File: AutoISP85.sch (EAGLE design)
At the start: 4 parts, among them J1 MCU, J2 BOARD, U1 ATTINY85, U2 BOARD

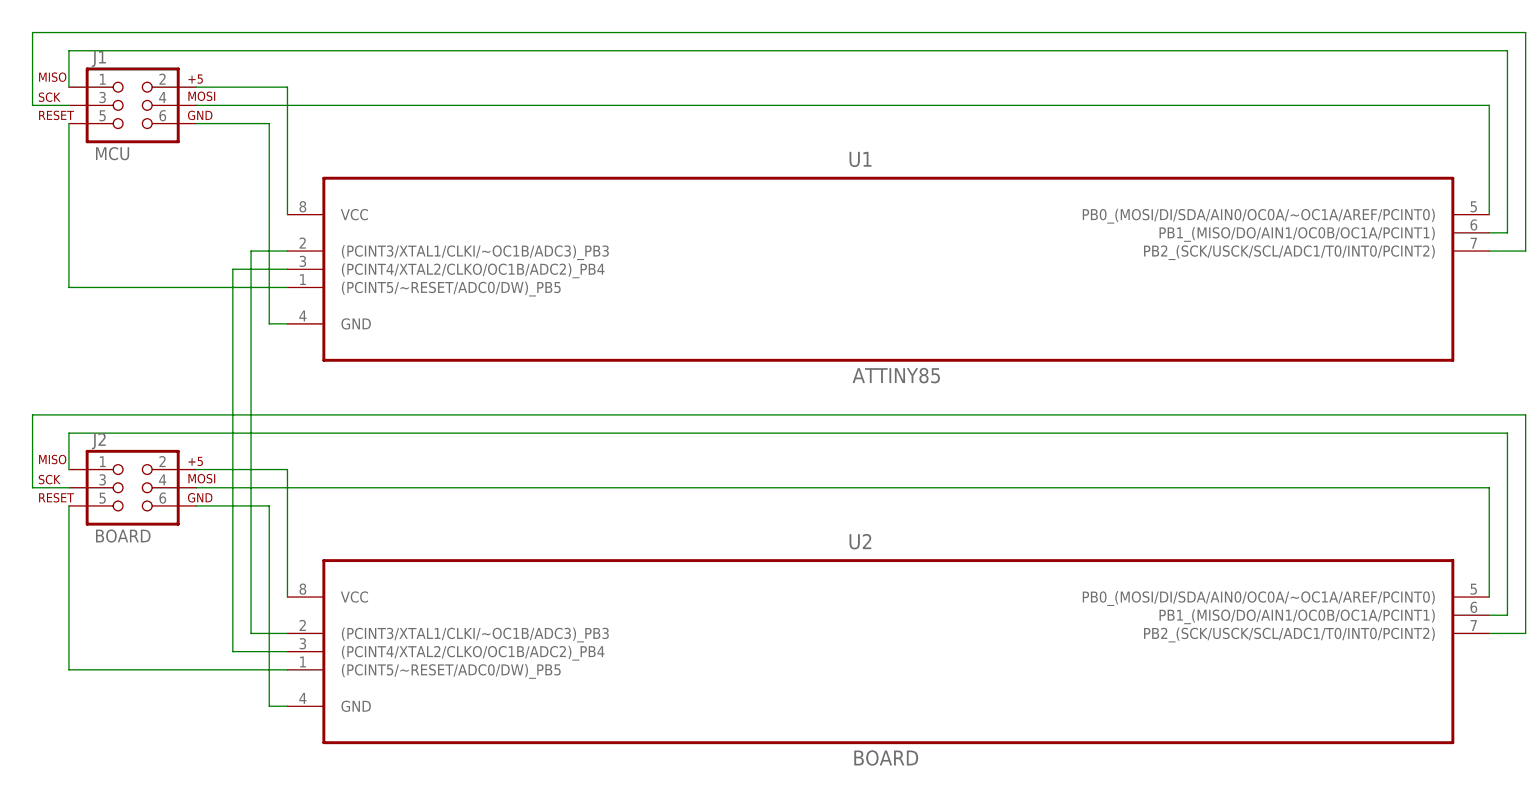
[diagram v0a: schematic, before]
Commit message: Revise boards for better labelling and sane orientation, add AutoISP328
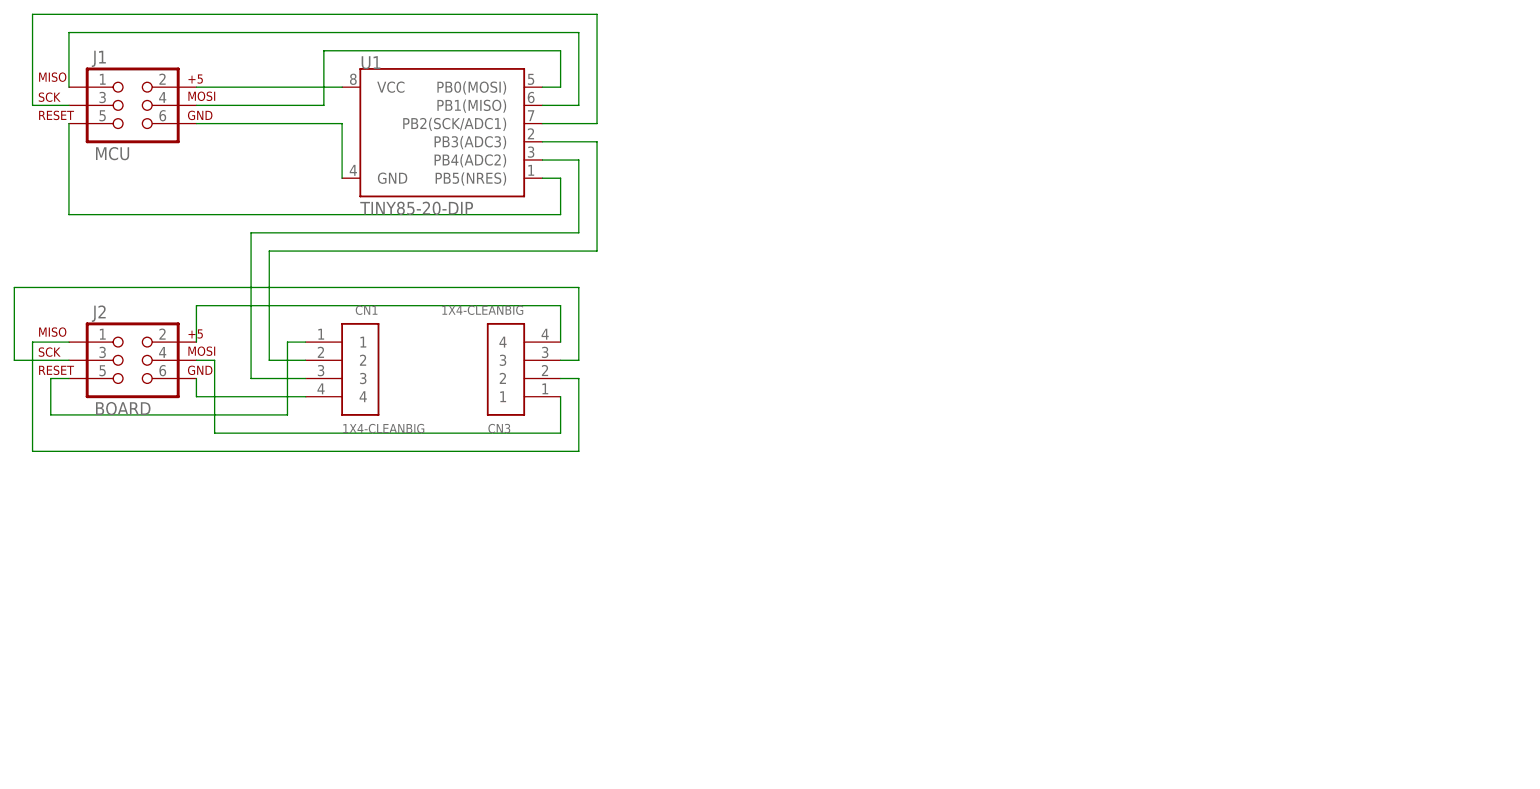
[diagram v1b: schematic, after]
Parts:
- removed U2: BOARD, Atmel_By_element14_Batch_1-00:ATTINY85-20PU
- added CN1, CN3: 1X4-CLEANBIG, adafruit:1X4-CLEANBIG
- U1: value ATTINY85 -> TINY85-20-DIP; device Atmel_By_element14_Batch_1-00:ATTINY85-20PU -> SparkFun-DigitalIC:ATTINY45TINY85-20-DIP
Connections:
- removed net N$13: U1.(PCINT3/XTAL1/CLKI/~OC1B/ADC3)_PB3, U2.(PCINT3/XTAL1/CLKI/~OC1B/ADC3)_PB3
- removed net N$14: U1.(PCINT4/XTAL2/CLKO/OC1B/ADC2)_PB4, U2.(PCINT4/XTAL2/CLKO/OC1B/ADC2)_PB4
- new net N$15: J1.1, U1.PB1(MISO)
- new net N$16: J1.3, U1.PB2(SCK/ADC1)
- net N$1: now also U1.PB5(NRES); no longer U1.(PCINT5/~RESET/ADC0/DW)_PB5
- net N$10: now also CN3.2, J2.1; no longer J2.4, U2.PB0_(MOSI/DI/SDA/AIN0/OC0A/~OC1A/AREF/PCINT0)
- net N$11: now also CN3.3, J2.3; no longer J2.1, U2.PB1_(MISO/DO/AIN1/OC0B/OC1A/PCINT1)
- net N$12: now also CN3.4, J2.2; no longer J2.3, U2.PB2_(SCK/USCK/SCL/ADC1/T0/INT0/PCINT2)
- net N$4: now also U1.PB0(MOSI); no longer U1.PB0_(MOSI/DI/SDA/AIN0/OC0A/~OC1A/AREF/PCINT0)
- net N$5: now also CN1.1, J2.5; no longer J1.1, U1.PB1_(MISO/DO/AIN1/OC0B/OC1A/PCINT1)
- net N$6: now also CN1.2, U1.PB3(ADC3); no longer J1.3, U1.PB2_(SCK/USCK/SCL/ADC1/T0/INT0/PCINT2)
- net N$7: now also CN1.3, U1.PB4(ADC2); no longer J2.5, U2.(PCINT5/~RESET/ADC0/DW)_PB5
- net N$8: now also CN1.4, J2.6; no longer J2.2, U2.VCC
- net N$9: now also CN3.1, J2.4; no longer J2.6, U2.GND
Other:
- moved on the sheet: J2
